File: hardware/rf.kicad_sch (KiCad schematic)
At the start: 17 parts, among them IC6 SI4468-A2A-IMR, Y1 TG2520SMN_30.000M-MCGNNM0

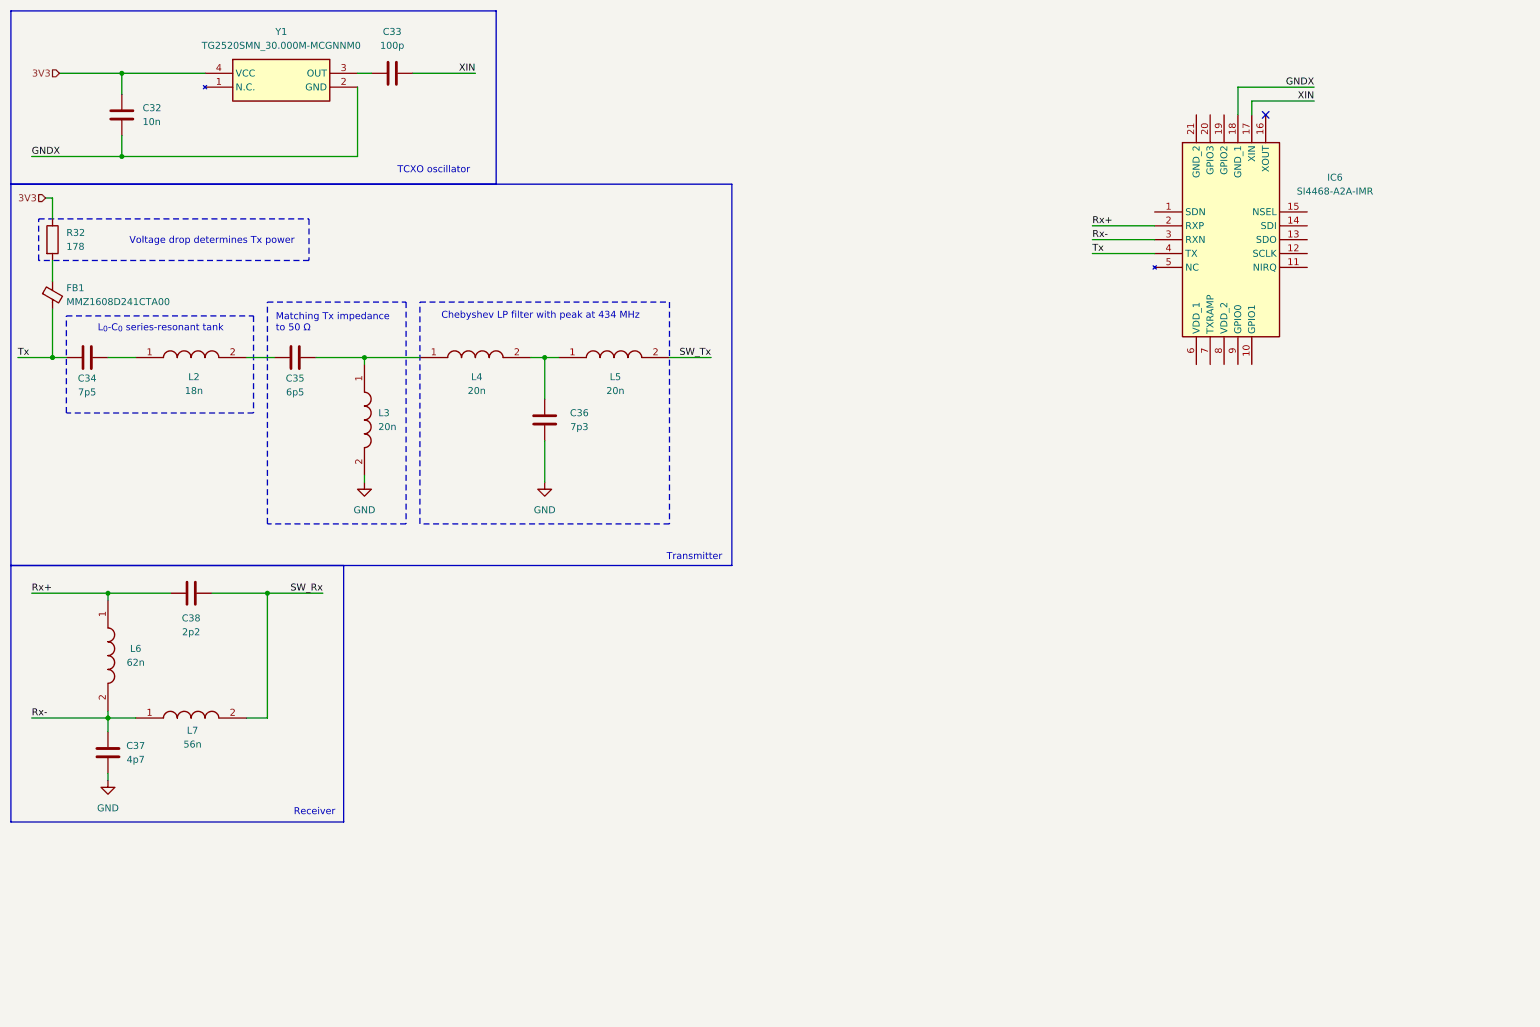
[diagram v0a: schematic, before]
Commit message: Done?
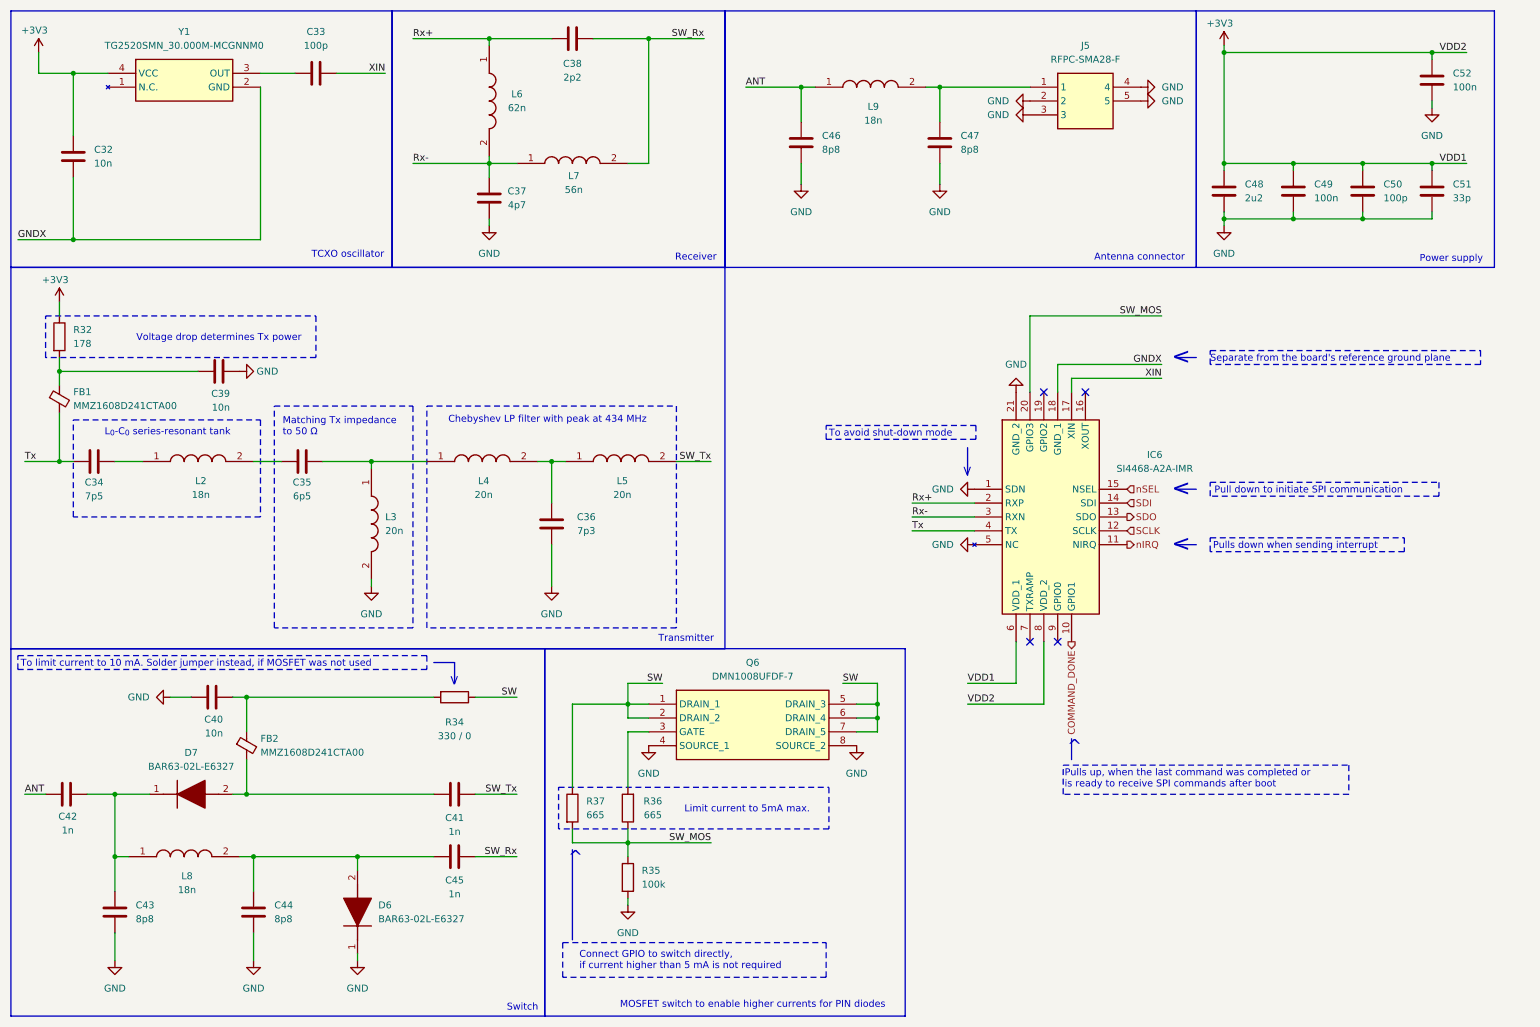
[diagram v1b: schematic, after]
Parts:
- added C39, C40: 10n, Capacitor_SMD:C_0402_1005Metric, symbol Device:C
- added C41, C42, C45: 1n, Capacitor_SMD:C_0402_1005Metric, symbol Device:C
- added C43, C44, C46, C47: 8p8, Capacitor_SMD:C_0402_1005Metric, symbol Device:C
- added C48: 2u2, Capacitor_SMD:C_0805_2012Metric, symbol Device:C
- added C49: 100n, Capacitor_SMD:C_0805_2012Metric, symbol Device:C
- added C50: 100p, Capacitor_SMD:C_0603_1608Metric, symbol Device:C
- added C51: 33p, Capacitor_SMD:C_0402_1005Metric, symbol Device:C
- added C52: 100n, Capacitor_SMD:C_0402_1005Metric, symbol Device:C
- added D6, D7: BAR63-02L-E6327, BAR6302LE6327, symbol SamacSys_Parts:BAR63-02L-E6327
- added FB2: MMZ1608D241CTA00, SamacSys_Parts:BEADC1608X95N, symbol Device:FerriteBead_Small
- added J5: RFPC-SMA28-F, RFPCSMA28F, symbol SamacSys_Parts:RFPC-SMA28-F
- added L8, L9: 18n, LQW15CNR20J00B, symbol SamacSys_Parts:LQW15AN20NG00D
- added Q6: DMN1008UFDF-7, DMN1008UFDF7, symbol SamacSys_Parts:DMN1008UFDF-7
- added R34: 330 / 0, Resistor_SMD:R_0402_1005Metric, symbol Device:R
- added R35: 100k, Resistor_SMD:R_0402_1005Metric, symbol Device:R
- added R36, R37: 665, Resistor_SMD:R_0402_1005Metric, symbol Device:R
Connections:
- net 3V3 is gone; now on net +3V3: C32.1, R32.1, Y1.4 (VCC)
- net GND: now also IC6.1 (SDN), IC6.21 (GND_2), IC6.5 (NC), C39.1, C40.2, C43.2, C44.2, C46.2, C47.2, C48.2, C49.2, C50.2, C51.2, C52.2, D6.1 (K), J5.2, J5.3, J5.4, J5.5, Q6.4 (SOURCE_1), Q6.8 (SOURCE_2), R35.2
- net SW_Rx: now also C45.2
- net SW_Tx: now also C41.2
- net at FB1.1, R32.2: now also C39.2
- net COMMAND_DONE: now reaches IC6.10 (GPIO1)
- net nIRQ: now reaches IC6.11 (NIRQ)
- net SCLK: now reaches IC6.12 (SCLK)
- net SDO: now reaches IC6.13 (SDO)
- net SDI: now reaches IC6.14 (SDI)
- net nSEL: now reaches IC6.15 (NSEL)
- net SW_MOS: now reaches IC6.20 (GPIO3)
- net SW_MOS: now also R35.1, R36.1, R37.2
- net +3V3: now reaches IC6.6 (VDD_1)
- net +3V3: now also IC6.8 (VDD_2), C48.1, C49.1, C50.1, C51.1, C52.1
- new net: Q6.3 (GATE), R36.2
- new net: C47.1, J5.1, L9.2
- new net: C44.1, C45.1, D6.2 (A), L8.2
- new net: C42.2, C43.1, D7.1 (K), L8.1
- new net: C41.1, D7.2 (A), FB2.2
- new net: C40.1, FB2.1, R34.2
- new net ANT: C42.1, C46.1, L9.1
- new net SW: Q6.1 (DRAIN_1), Q6.2 (DRAIN_2), Q6.5 (DRAIN_3), Q6.6 (DRAIN_4), Q6.7 (DRAIN_5), R34.1, R37.1
- no-connect marks 1 -> 4
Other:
- note added: "<"
- note added: "Antenna connector"
- note added: "Connect GPIO to switch directly, if current higher than 5 mA is not required"
- note added: "Limit current to 5mA max."
- note added: "MOSFET switch to enable higher currents for PIN diodes"
- note added: "Power supply"
- note added: "Pull down to initiate SPI communication"
- note added: "Pulls down when sending interrupt"
- note added: "Pulls up, when the last command was completed or is ready to receive SPI commands after boot"
- note added: "Separate from the board's reference ground plane"
- note added: "Switch"
- note added: "To avoid shut-down mode"
- note added: "To limit current to 10 mA. Solder jumper instead, if MOSFET was not used"
- note added: "V"
- note added: "^"
- moved on the sheet: C32, C33, C34, C35, C36, C37, C38, FB1, IC6, L2, L3, L4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
